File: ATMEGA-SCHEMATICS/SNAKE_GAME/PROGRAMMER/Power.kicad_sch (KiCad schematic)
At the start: 0 parts

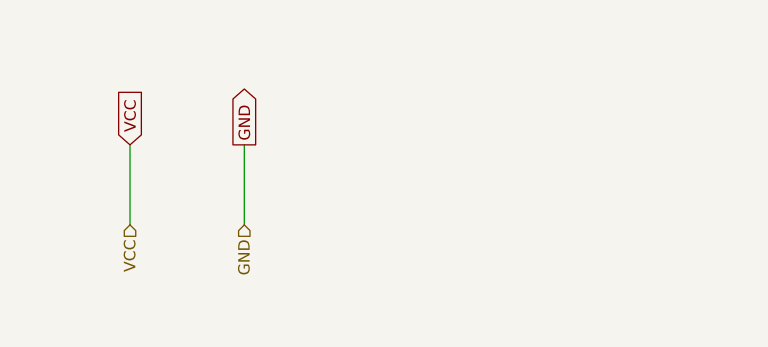
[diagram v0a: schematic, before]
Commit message: PWR_USBC_UART_ATMEGA8
Come back to Earth - Mac Miller
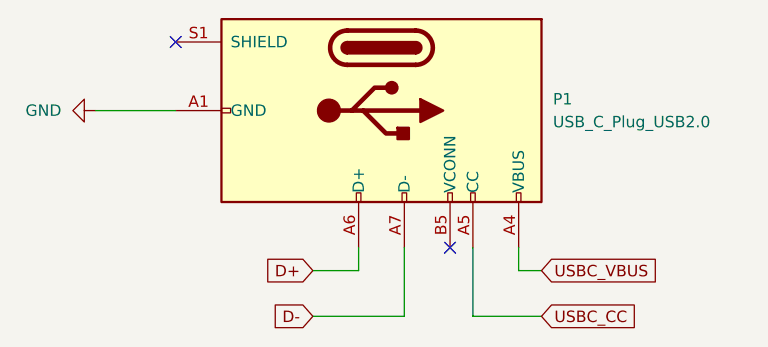
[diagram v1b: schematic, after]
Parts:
- added P1: USB_C_Plug_USB2.0, symbol Connector:USB_C_Plug_USB2.0
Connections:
- net GND: now also P1.A1 (GND), P1.A12 (GND), P1.B1 (GND), P1.B12 (GND)
- new net D+: P1.A6 (D+)
- new net D-: P1.A7 (D-)
- new net USBC_CC: P1.A5 (CC)
- new net USBC_VBUS: P1.A4 (VBUS), P1.A9 (VBUS), P1.B4 (VBUS), P1.B9 (VBUS)
- no-connect marks 0 -> 2
